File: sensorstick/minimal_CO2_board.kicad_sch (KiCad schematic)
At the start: 5 parts, among them J1 USB_A, U1 ESP32-C3_SUPERMINI

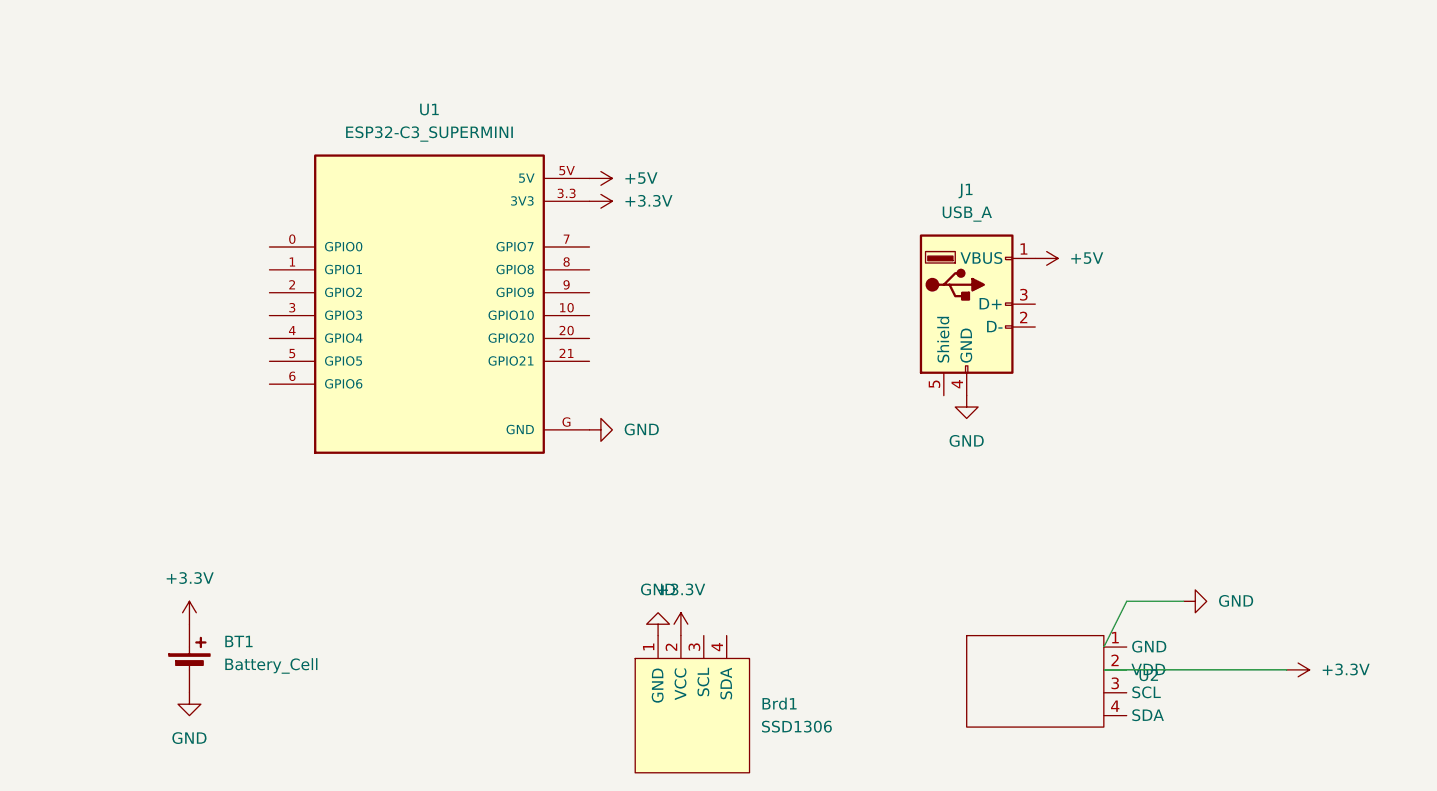
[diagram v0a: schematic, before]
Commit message: add stuff
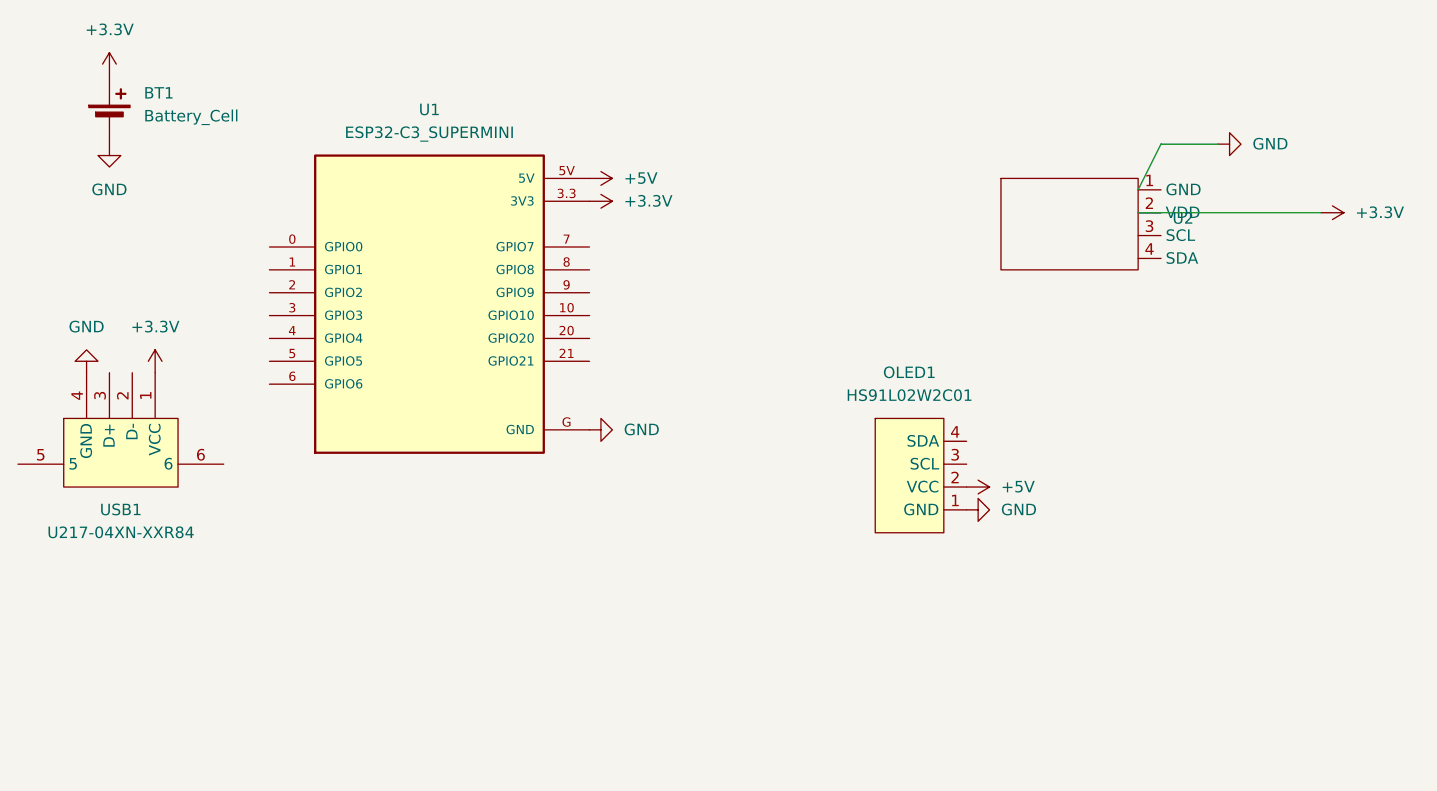
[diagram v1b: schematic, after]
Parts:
- removed Brd1: SSD1306, CustomLibrary:128x64OLED, symbol CustomSymbols:SSD1306
- removed J1: USB_A, Connector_USB:USB_A_CNCTech_1001-011-01101_Horizontal, symbol Connector:USB_A
- added OLED1: HS91L02W2C01, CustomLibrary:OLED-TH_L38.0-W12.0_HS91L02W2C01, symbol CustomSymbols:HS91L02W2C01
- added USB1: U217-04XN-XXR84, CustomLibrary:USB-A-SMD_U217-041N-4BV81, symbol CustomSymbols:U217-04XN-XXR84
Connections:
- net +3.3V: now also USB1.1 (VCC)
- net +5V: now also OLED1.2 (VCC)
- net GND: now also OLED1.1 (GND), USB1.4 (GND)
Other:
- moved on the sheet: BT1, U2
